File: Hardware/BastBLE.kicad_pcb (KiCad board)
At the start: 2 copper layers, 50.8 x 22.9 mm, 39 parts, among them J1 Conn_Battery, J2 SWD, J3 Conn_left, J4 Conn_right, P1 USB_C_Plug_USB2.0, Q1 DMG3415U-7, SW1 RESET, U1 AP2112K-3.3, U2 E73-2G4M08S1C, U3 MCP73831-2-OT, U4 W25Q32JVSS, Y1 32Khz

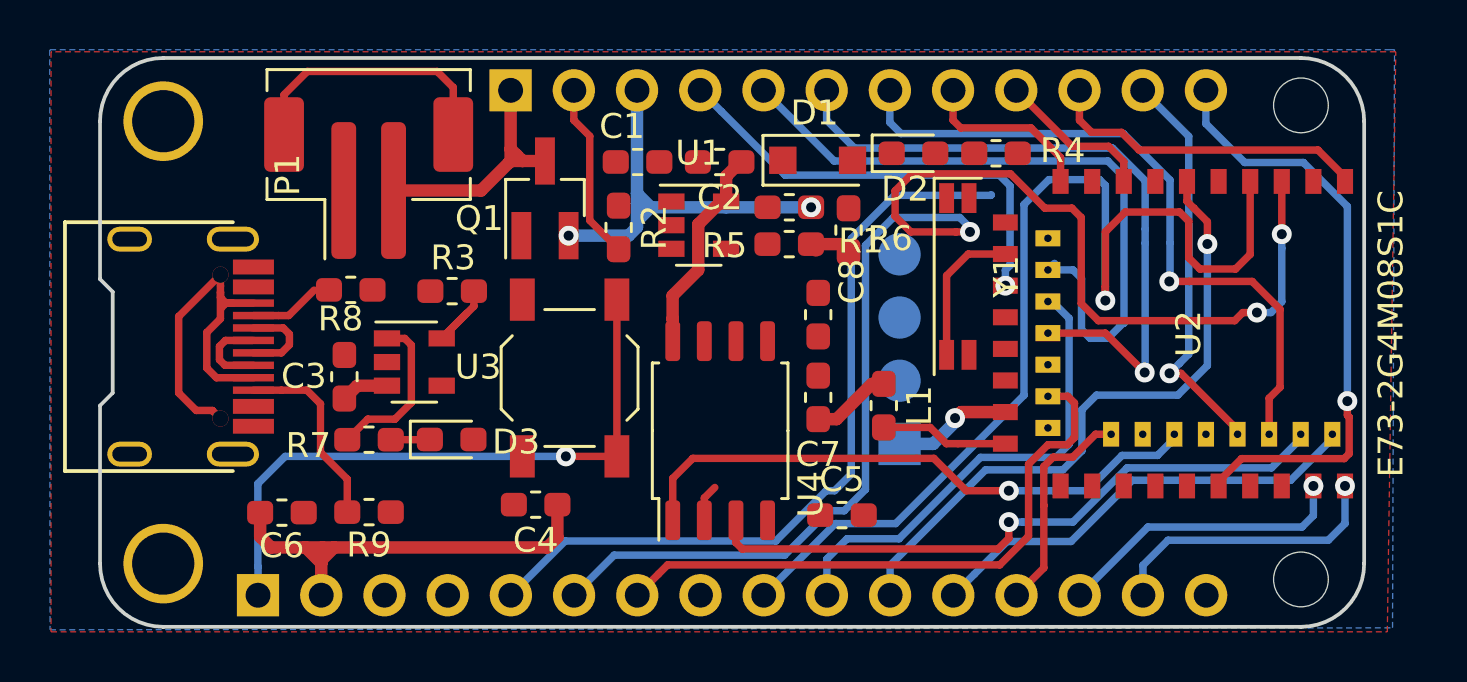
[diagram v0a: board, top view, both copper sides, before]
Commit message: erase traces, add note
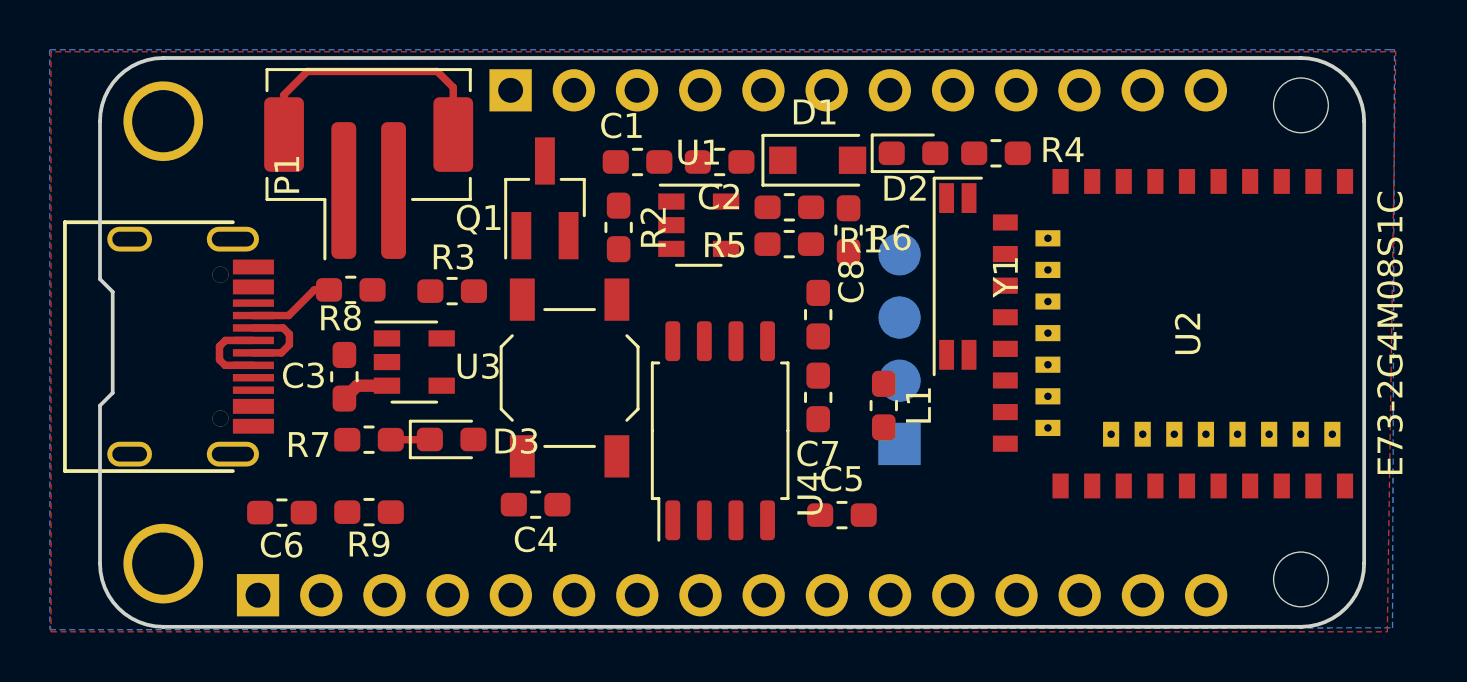
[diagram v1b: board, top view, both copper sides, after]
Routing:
- net /A1: track 58.0 -> 0.00 mm, vias 3 -> 0
- net /A4: track 44.3 -> 0.00 mm, vias 1 -> 0
- net +3V3: track 35.0 -> 0.00 mm, vias 1 -> 0
- net /A0: track 31.5 -> 0.00 mm
- net /D12: track 27.8 -> 0.00 mm
- net /D10: track 27.7 -> 0.00 mm, vias 1 -> 0
- net /D11: track 27.3 -> 0.00 mm, vias 1 -> 0
- net /QSPI_DATA2: track 26.1 -> 0.00 mm, vias 1 -> 0
- net /SCK: track 26.0 -> 0.00 mm, vias 1 -> 0
- net /RST: track 25.7 -> 0.00 mm, vias 1 -> 0
- net /A2: track 24.5 -> 0.00 mm
- net /SDA: track 24.3 -> 0.00 mm, vias 1 -> 0
- net /QSPI_CS: track 23.8 -> 0.00 mm, vias 1 -> 0
- net /A5: track 19.3 -> 0.00 mm
- net /D13: track 18.1 -> 0.00 mm, vias 1 -> 0
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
